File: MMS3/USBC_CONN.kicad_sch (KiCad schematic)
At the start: 7 parts, among them J800 USB_C_Receptacle_USB2.0_16P, U401 TPD2EUSB30DRTR-TP

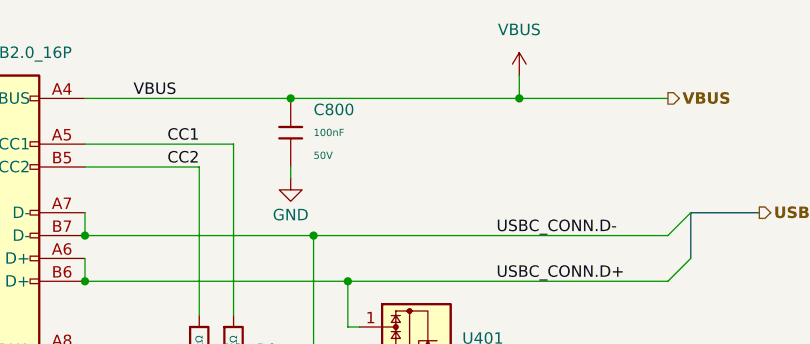
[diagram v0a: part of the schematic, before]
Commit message: prod ready
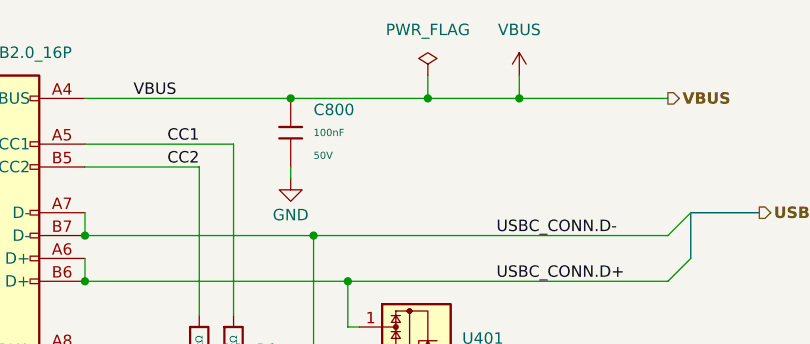
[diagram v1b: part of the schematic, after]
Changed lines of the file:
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@@
+	)
+	(junction
+		(at 153.67 73.66)
+		(diameter 0)
+		(color 0 0 0 0)
 	)
 	(junction
@@
 	(wire
 		(pts
+			(xy 153.67 71.12) (xy 153.67 73.66)
+		)
+		(stroke
+			(width 0)
+			(type default)
+		)
+	)
+	(wire
+		(pts
 			(xy 132.08 105.41) (xy 132.08 107.95)
 		)
@@
 	(wire
 		(pts
-			(xy 138.43 73.66) (xy 163.83 73.66)
+			(xy 138.43 73.66) (xy 153.67 73.66)
 		)
 		(stroke
@@
 		(pts
 			(xy 100.33 119.38) (xy 100.33 120.65)
+		)
+		(stroke
+			(width 0)
+			(type default)
+		)
+	)
+	(wire
+		(pts
+			(xy 153.67 73.66) (xy 163.83 73.66)
 		)
 		(stroke
@@
 					(unit 1)
 				)
+			)
+		)
+	)
+	(symbol
+		(lib_id "power:PWR_FLAG")
+		(at 153.67 71.12 0)
+		(unit 1)
+		(body_style 1)
+		(exclude_from_sim no)
+		(in_bom yes)
+		(on_board yes)
+		(in_pos_files yes)
+		(dnp no)
+		(fields_autoplaced yes)
+		(property "Reference" "#FLG02"
+			(at 153.67 69.215 0)
+			(hide yes)
+			(show_name no)
+			(do_not_autoplace no)
+			(effects
+				(font
+					(size 1.27 1.27)
+				)
+			)
+		)
+		(property "Value" "PWR_FLAG"
+			(at 153.67 66.04 0)
+			(show_name no)
+			(do_not_autoplace no)
+			(effects
+				(font
+					(size 1.27 1.27)
+				)
+			)
+		)
+		(property "Footprint" ""
+			(at 153.67 71.12 0)
+			(hide yes)
+			(show_name no)
+			(do_not_autoplace no)
+			(effects
+				(font
+					(size 1.27 1.27)
+				)
+			)
+		)
+		(property "Datasheet" ""
+			(at 153.67 71.12 0)
+			(hide yes)
+			(show_name no)
+			(do_not_autoplace no)
+			(effects
+				(font
+					(size 1.27 1.27)
+				)
+			)
+		)
+		(property "Description" "Special symbol for telling ERC where power comes from"
+			(at 153.67 71.12 0)
+			(hide yes)
+			(show_name no)
+			(do_not_autoplace no)
+			(effects
+				(font
+					(size 1.27 1.27)
+				)
+			)
+		)
+		(pin "1"
+		)
+		(instances
+			(project "MMS3"
+				(path "/712cea22-140d-4c92-923f-f4998caf3ecd/6293ce90-9b00-41f8-95cd-8a2592163f0a"
+					(reference "#FLG02")
+					(unit 1)
+				)
